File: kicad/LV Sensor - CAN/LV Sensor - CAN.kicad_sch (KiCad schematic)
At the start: 9 parts, among them J2 Conn_01x09_Pin, U1 MCP2518FD-xJHA, U2 DSC1001DL5-020.0000T, U5 ATA6561-GAQW-N

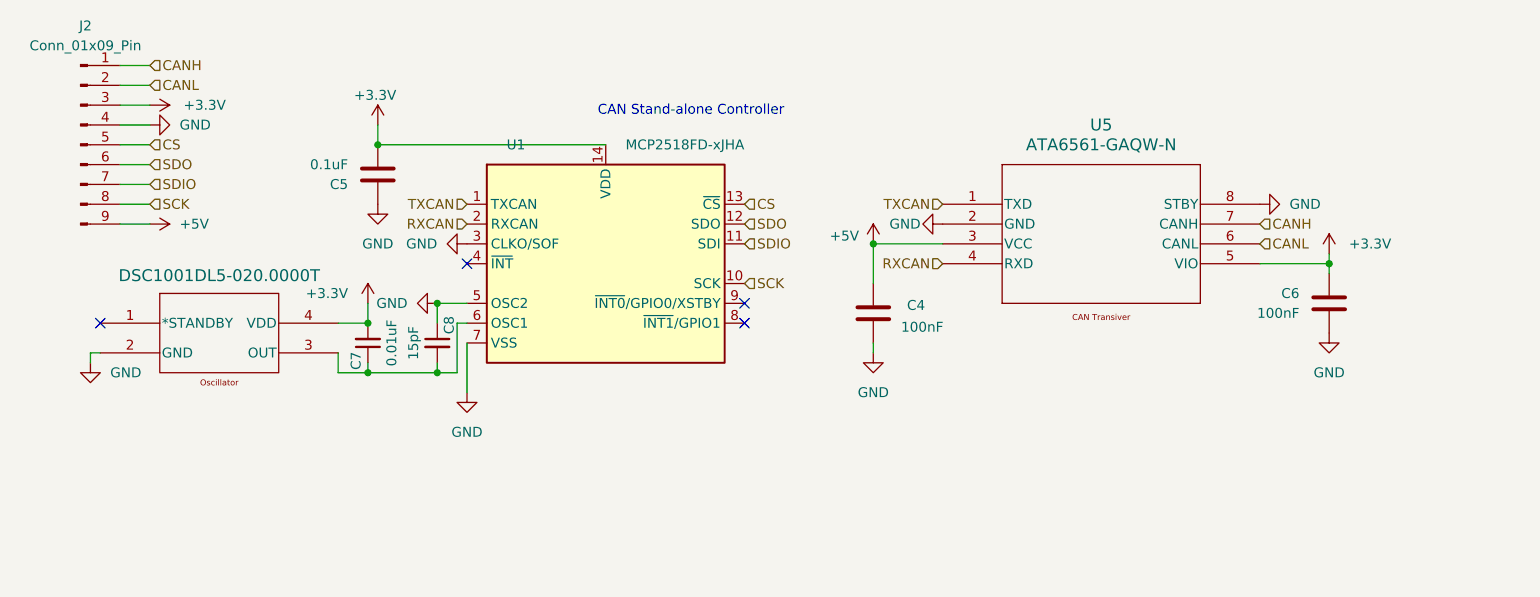
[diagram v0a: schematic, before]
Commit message: 09-10-25
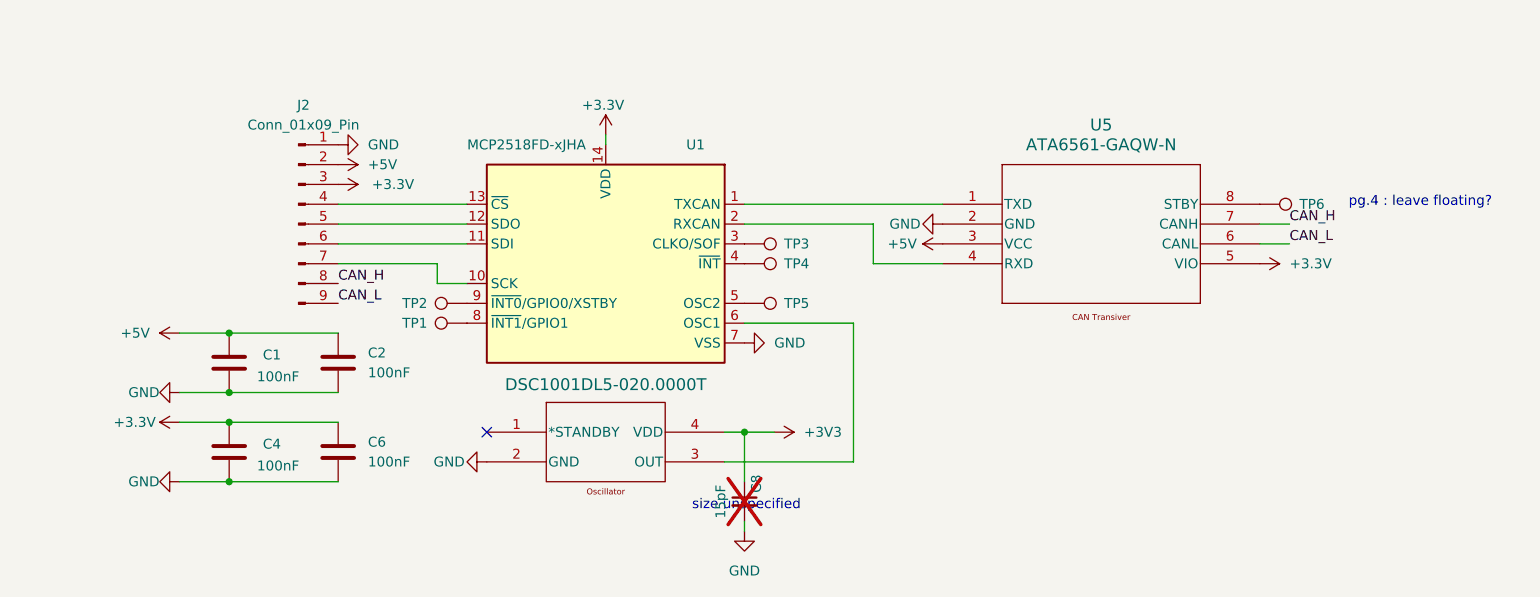
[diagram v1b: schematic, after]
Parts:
- removed C5: 0.1uF, Capacitor_SMD:C_1206_3216Metric_Pad1.33x1.80mm_HandSolder, symbol Device:C
- removed C7: 0.01uF, Capacitor_SMD:C_1206_3216Metric_Pad1.33x1.80mm_HandSolder, symbol Device:C_Small
- added C1, C2: 100nF, Capacitor_SMD:C_1206_3216Metric_Pad1.33x1.80mm_HandSolder, symbol Device:C
- added TP1, TP2, TP3, TP4, TP5, TP6: TestPoint, Connector_Pin:Pin_D1.0mm_L10.0mm, symbol Connector:TestPoint
- C8: now not fitted; now left out of the parts list
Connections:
- net +3.3V: now also C4.1; no longer U2.4 (VDD)
- net +5V: now also J2.2 (Pin_2), C1.1, C2.1; no longer C4.1, J2.9 (Pin_9)
- net GND: now also C8.2, J2.1 (Pin_1), C1.2, C2.2; no longer C8.1, J2.4 (Pin_4), U1.3 (CLKO/SOF), U1.5 (OSC2), U5.8 (STBY)
- net at U1.6 (OSC1), U2.3 (OUT): no longer C8.2
- net at U1.4 (~{INT}): now also TP4.1
- net at U1.8 (~{INT1}/GPIO1): now also TP1.1
- net at U1.9 (~{INT0}/GPIO0/XSTBY): now also TP2.1
- net CANH renamed CAN_H
- net CAN_H: now also J2.8 (Pin_8); no longer J2.1 (Pin_1)
- net CANL renamed CAN_L
- net CAN_L: now also J2.9 (Pin_9); no longer J2.2 (Pin_2)
- net CS: no longer names the net of U1.13 (~{CS})
- net CS: now also J2.4 (Pin_4); no longer J2.5 (Pin_5)
- net RXCAN: no longer names the net of U1.2 (RXCAN), U5.4 (RXD)
- net SCK: no longer names the net of U1.10 (SCK)
- net SCK: now also J2.7 (Pin_7); no longer J2.8 (Pin_8)
- net SDIO: no longer names the net of U1.11 (SDI)
- net SDIO: now also J2.6 (Pin_6); no longer J2.7 (Pin_7)
- net SDO: no longer names the net of U1.12 (SDO)
- net SDO: now also J2.5 (Pin_5); no longer J2.6 (Pin_6)
- net TXCAN: no longer names the net of U1.1 (TXCAN), U5.1 (TXD)
- new net: TP6.1, U5.8 (STBY)
- new net: TP5.1, U1.5 (OSC2)
- new net: TP3.1, U1.3 (CLKO/SOF)
- new net +3V3: C8.1, U2.4 (VDD)
- no-connect marks 4 -> 1
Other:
- note added: "pg.4 : leave floating?"
- note added: "size unspecified"
- note removed: "CAN Stand-alone Controller"
- moved on the sheet: C4, C6, J2
